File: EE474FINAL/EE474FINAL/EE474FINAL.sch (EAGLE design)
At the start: 24 parts, among them U1 TM4C123_DEVICE, U4 3.3V

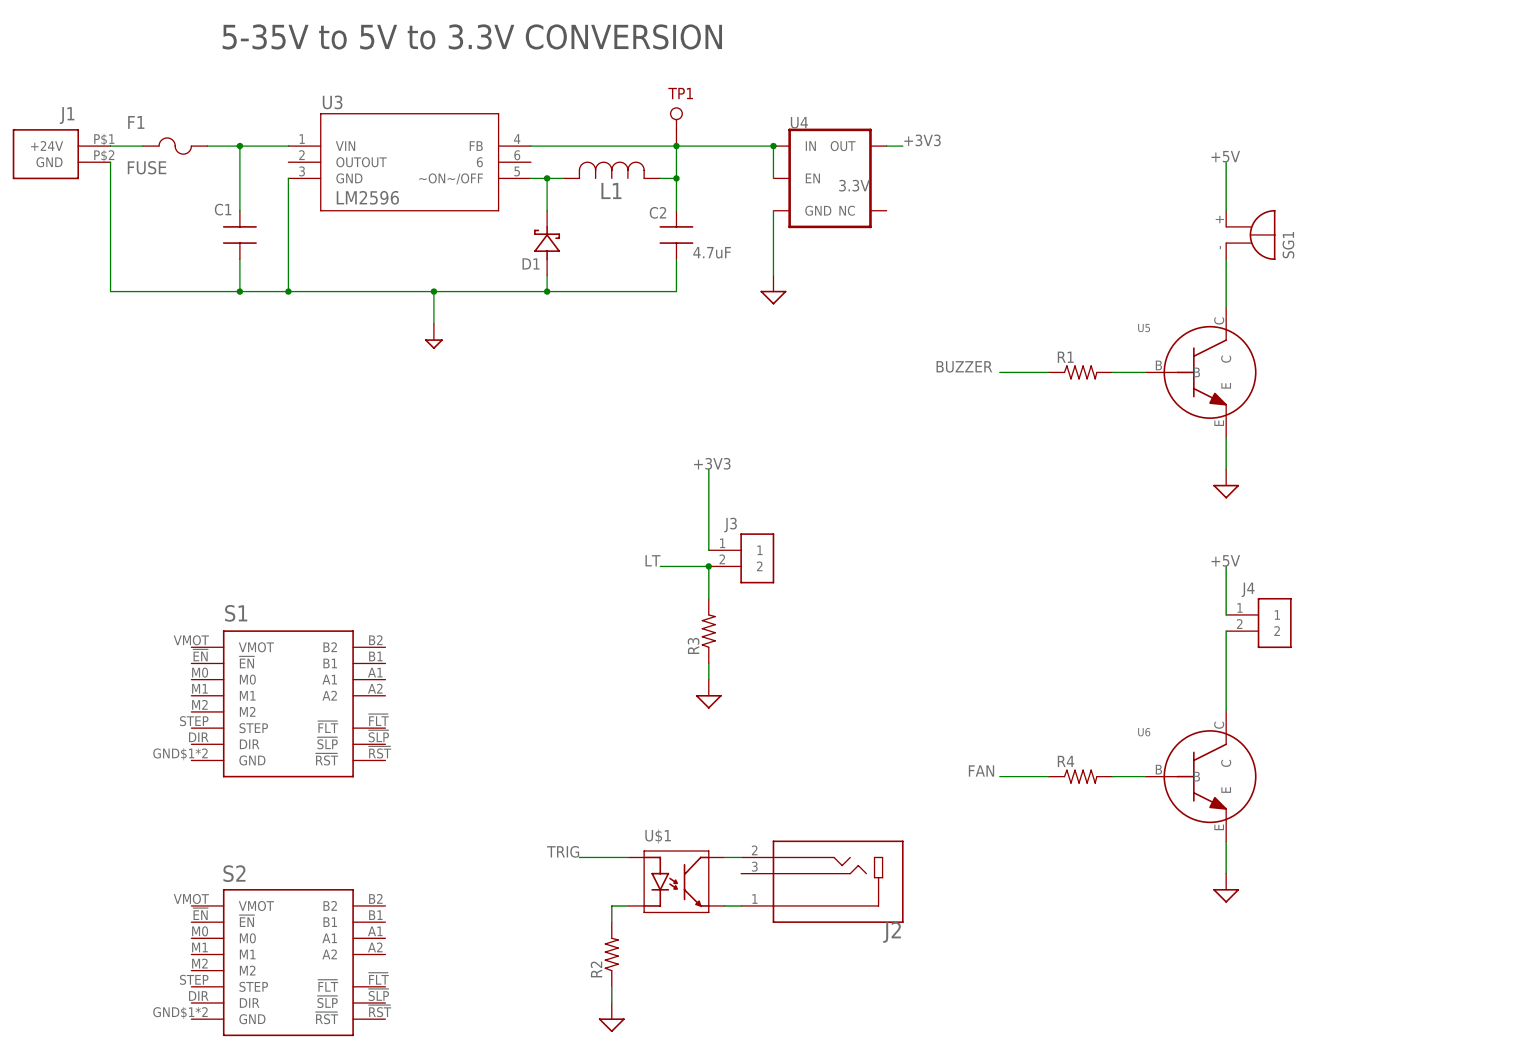
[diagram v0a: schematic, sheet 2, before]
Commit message: Ready for layout
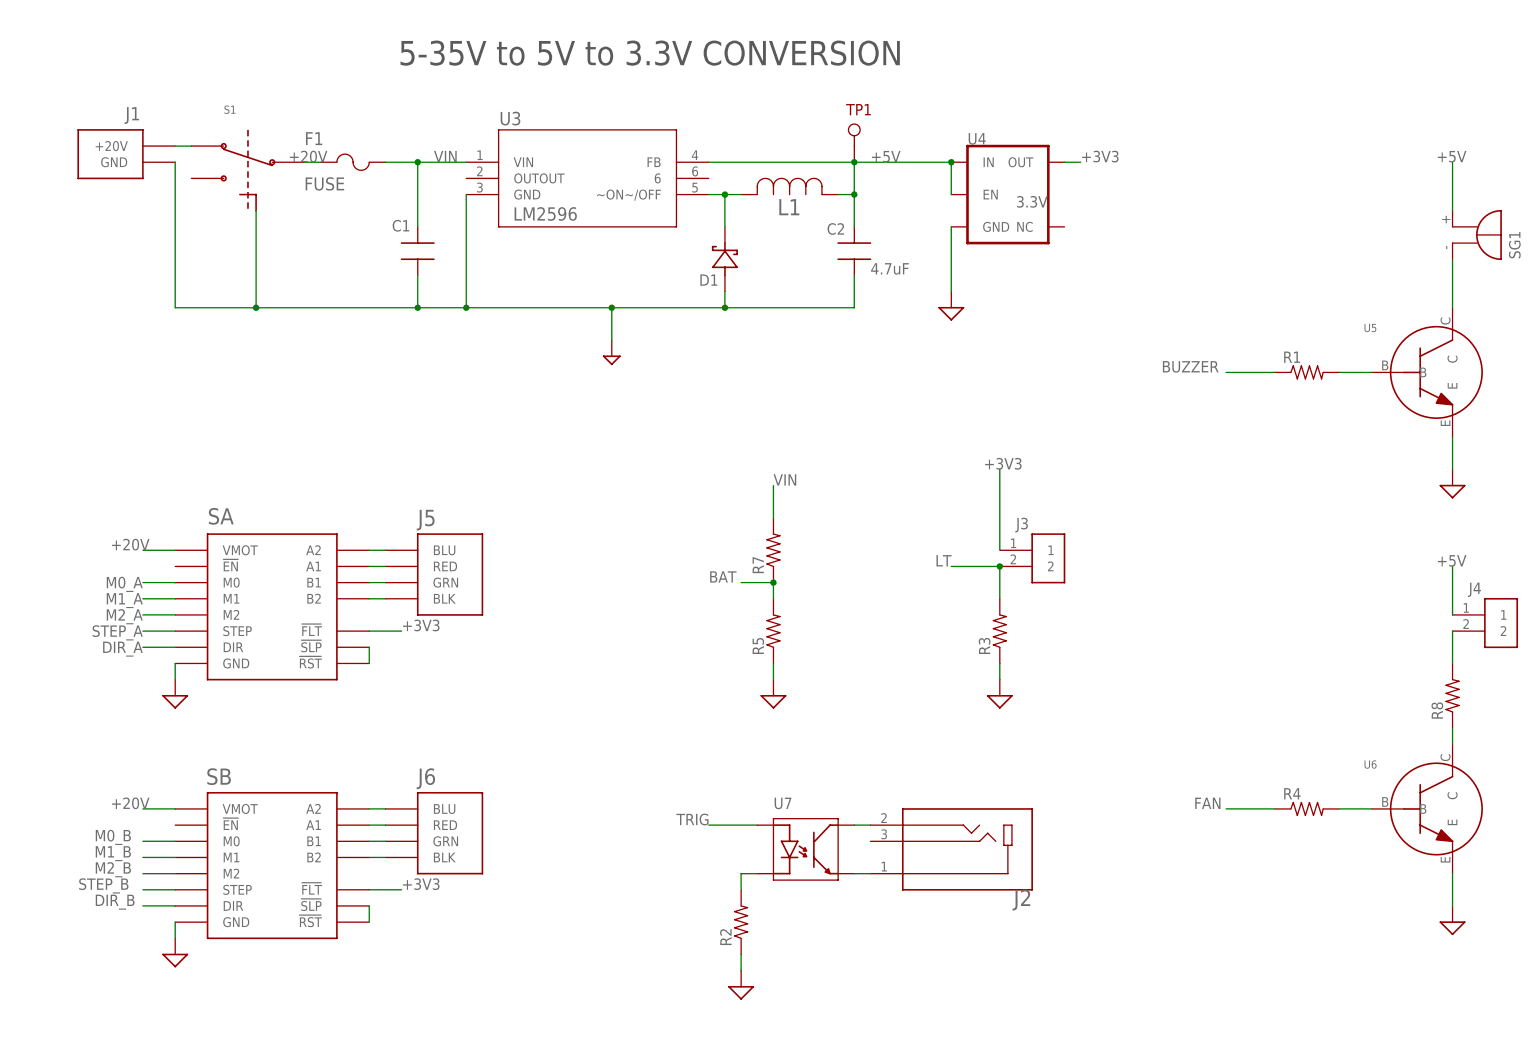
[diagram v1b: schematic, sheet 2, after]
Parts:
- removed S2: (no value), MICROCONTROLLER:DRV8825
- removed U$1: (no value), FillControl:OPTOISOLATOR
- added C10: 2.2uF, MICROCONTROLLER:CAPACITOR
- added C11, C12, C13, C14, C15, C16, C7, C8: .1uF, MICROCONTROLLER:CAPACITOR
- added C3, C4: 24pF, MICROCONTROLLER:CAPACITOR
- added C5, C6: 10pF, MICROCONTROLLER:CAPACITOR
- added C9: 1uF, MICROCONTROLLER:CAPACITOR
- added GND, PA2, PA3, PA4, PA5: (no value), MICROCONTROLLER:TESTPOINT
- added J5, J6: (no value), MICROCONTROLLER:4POS_MOLEXVERT
- added J7: (no value), MICROCONTROLLER:6POS_JST
- added R5, R7, R8: (no value), rcl:R-US_R0402
- added R6: 1M, MICROCONTROLLER:RESISTOR
- added SA, SB: (no value), MICROCONTROLLER:DRV8825
- added U7: (no value), FillControl:OPTOISOLATOR
- added Y1: 32kHz, MICROCONTROLLER:32KHZ_OSCILATOR
- added Y2: Y2, MICROCONTROLLER:16MHZ_OSCILLATOR
- S1: device MICROCONTROLLER:DRV8825 -> MICROCONTROLLER:SLIDESWITCH
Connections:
- removed net +24V: F1.1, J1.+24V
- removed net +VBUS: U4.EN, U4.IN
- new net !RST: U1.!RST
- new net !WAKE: R6.2, U1.!WAKE
- new net +20V: F1.1, S1.2, SA.VMOT, SB.VMOT
- new net BAT: R5.2, R7.1, U1.PE3
- new net CTS: U2.UART_CTS
- new net DIR_A: SA.DIR, U1.PD4
- new net DIR_B: SB.DIR, U1.PF4
- new net M0_A: SA.M0, U1.PD0
- new net M0_B: SB.M0, U1.PF0
- new net M1_A: SA.M1, U1.PD1
- new net M1_B: SB.M1, U1.PF1
- new net M2_A: SA.M2, U1.PD2
- new net M2_B: SB.M2, U1.PF2
- new net N$10: J5.GRN, SA.B1
- new net N$11: J5.BLK, SA.B2
- new net N$12: J6.BLU, SB.A2
- new net N$13: J6.RED, SB.A1
- new net N$14: J6.GRN, SB.B1
- new net N$15: J6.BLK, SB.B2
- new net N$16: SB.!RST, SB.!SLP
- new net N$17: SA.!RST, SA.!SLP
- new net N$19: J1.+20V, S1.1
- new net N$20: R8.1, U6.C
- new net N$21: PA3.P$1, U1.PA3/SSI0FSS
- new net N$38: C3.1, U1.OSC0, Y1.2
- new net N$39: C4.2, U1.OSC1, Y1.1
- new net N$40: C3.2, C4.1, U1.GNDX
- new net N$41: C5.2, U1.XOSC0, Y2.2
- new net N$42: C6.1, U1.XOSC1, Y2.1
- new net N$8: J5.BLU, SA.A2
- new net N$9: J5.RED, SA.A1
- new net PA2: PA2.P$1, U1.PA2/SSI0CLK
- new net PA4: PA4.P$1, U1.PA4/SSI0RX
- new net PA5: PA5.P$1, U1.PA5/SSI0TX
- new net RTS: U2.UART_RTS
- new net RX-1: U1.PB1/USB0VBUS, U2.UART_RX
- new net RXD: J7.1, U1.PA0/U0RX
- new net STEP_A: SA.STEP, U1.PD3
- new net STEP_B: SB.STEP, U1.PF3
- new net TCK: J7.3, U1.PC0/TCK/SWCLK
- new net TDI: J7.5, U1.PC2/TDI
- new net TDO: J7.6, U1.PC3/TDO/SWO
- new net TMS: J7.4, U1.PC1/TMS/SWDIO
- new net TX-0: U1.PB0/USB0ID, U2.UART_TX
- new net TXD: J7.2, U1.PA1/U0TX
- new net VDDC: C10.2, C7.2, C8.2, C9.2, U1.VDDC, U1.VDDC_2
- net +3V3: now also C11.2, C12.2, C13.2, C14.2, C15.2, C16.2, SA.!FLT, SB.!FLT, U1.VBAT, U1.VDD, U1.VDDA, U1.VDD_2, U1.VDD_3, U1.VDD_4, U2.VDD
- net +5V: now also R6.1, U4.EN, U4.IN
- net BUZZER: now also U1.PA6
- net FAN: now also U1.PA7
- net GND: now also C10.1, C11.1, C12.1, C13.1, C14.1, C15.1, C16.1, C5.1, C6.2, C7.1, C8.1, C9.1, GND.P$1, R5.1, S1.GND, SA.GND, SB.GND, U1.GND, U1.GNDA, U1.GND_2, U1.GND_3, U1.GND_4, U2.GND
- net LT: now also U1.PE2
- net N$3: now also U7.4; no longer U$1.4
- net N$4: now also U7.3; no longer U$1.3
- net N$5: now also R8.2; no longer U6.C
- net N$6: now also U7.2; no longer U$1.2
- net TRIG: now also U1.PB5, U7.1; no longer U$1.1
- net VIN: now also R7.2
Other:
- moved on the sheet: C1, C2, D1, F1, J2, J3, J4, L1, R1, R2, R3, R4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
